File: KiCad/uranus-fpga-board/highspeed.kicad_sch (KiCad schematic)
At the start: 1 part, among them J1 ASP-134488-01

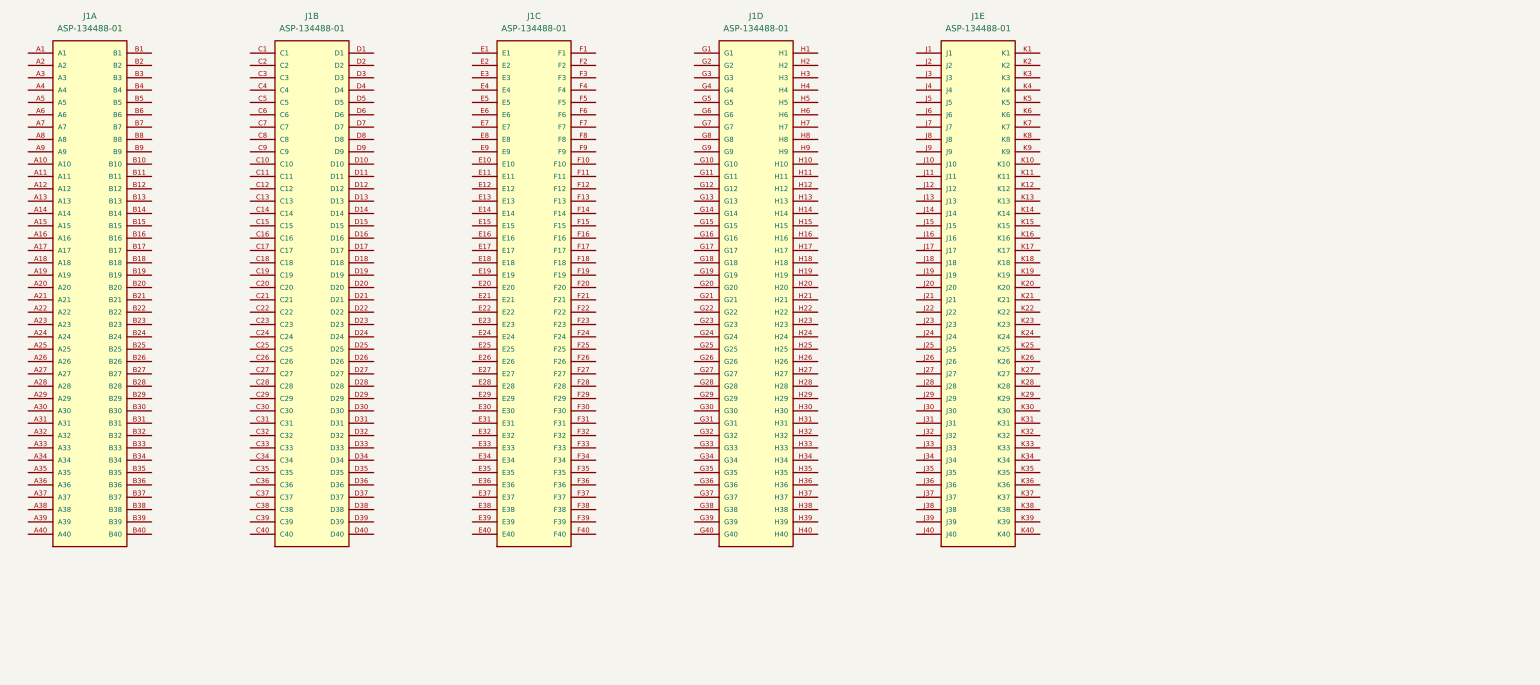
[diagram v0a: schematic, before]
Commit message: up to dating
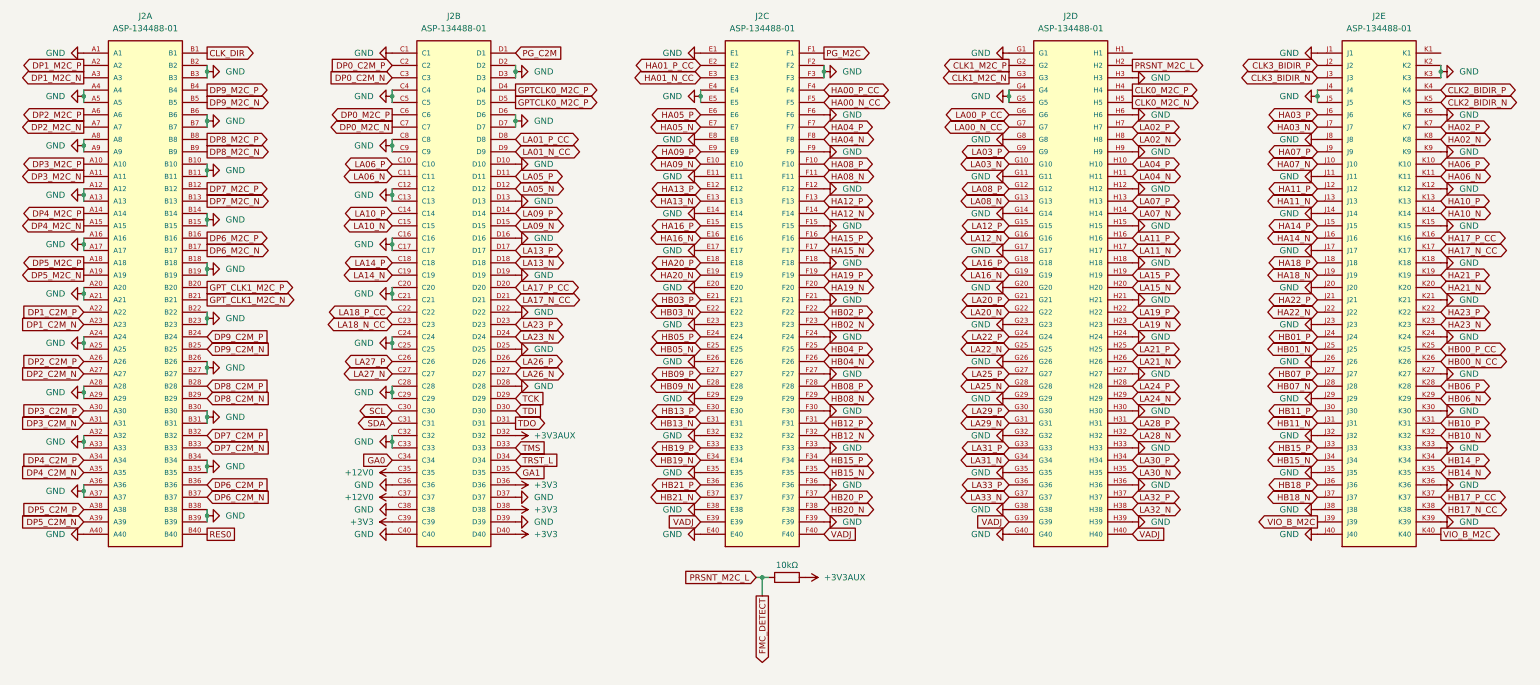
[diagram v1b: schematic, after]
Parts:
- removed J1: ASP-134488-01, FMC-HPC:SAMTEC_ASP-134488-01, symbol ASP-134488-01:ASP-134488-01
- added J2: ASP-134488-01, ASP-134488-01:SAMTEC_ASP-134488-01, symbol ASP-134488-01:ASP-134488-01
- added R14: 10kΩ, ASP-134488-01:SAMTEC_ASP-134488-01, symbol Device:R
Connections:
- new net +12V0: J2.C35, J2.C37
- new net +3V3: J2.C39, J2.D36, J2.D38, J2.D40
- new net +3V3AUX: J2.D32, R14.2
- new net CLK0_M2C_N: J2.H5
- new net CLK0_M2C_P: J2.H4
- new net CLK1_M2C_N: J2.G3
- new net CLK1_M2C_P: J2.G2
- new net CLK2_BIDIR_N: J2.K5
- new net CLK2_BIDIR_P: J2.K4
- new net CLK3_BIDIR_N: J2.J3
- new net CLK3_BIDIR_P: J2.J2
- new net CLK_DIR: J2.B1
- new net DP0_C2M_N: J2.C3
- new net DP0_C2M_P: J2.C2
- new net DP0_M2C_N: J2.C7
- new net DP0_M2C_P: J2.C6
- new net DP1_C2M_N: J2.A23
- new net DP1_C2M_P: J2.A22
- new net DP1_M2C_N: J2.A3
- new net DP1_M2C_P: J2.A2
- new net DP2_C2M_N: J2.A27
- new net DP2_C2M_P: J2.A26
- new net DP2_M2C_N: J2.A7
- new net DP2_M2C_P: J2.A6
- new net DP3_C2M_N: J2.A31
- new net DP3_C2M_P: J2.A30
- new net DP3_M2C_N: J2.A11
- new net DP3_M2C_P: J2.A10
- new net DP4_C2M_N: J2.A35
- new net DP4_C2M_P: J2.A34
- new net DP4_M2C_N: J2.A15
- new net DP4_M2C_P: J2.A14
- new net DP5_C2M_N: J2.A39
- new net DP5_C2M_P: J2.A38
- new net DP5_M2C_N: J2.A19
- new net DP5_M2C_P: J2.A18
- new net DP6_C2M_N: J2.B37
- new net DP6_C2M_P: J2.B36
- new net DP6_M2C_N: J2.B17
- new net DP6_M2C_P: J2.B16
- new net DP7_C2M_N: J2.B33
- new net DP7_C2M_P: J2.B32
- new net DP7_M2C_N: J2.B13
- new net DP7_M2C_P: J2.B12
- new net DP8_C2M_N: J2.B29
- new net DP8_C2M_P: J2.B28
- new net DP8_M2C_N: J2.B9
- new net DP8_M2C_P: J2.B8
- new net DP9_C2M_N: J2.B25
- new net DP9_C2M_P: J2.B24
- new net DP9_M2C_N: J2.B5
- new net DP9_M2C_P: J2.B4
- new net FMC_DETECT: J2.H2, R14.1
- new net GA0: J2.C34
- new net GA1: J2.D35
- new net GND: J2.A1, J2.A12, J2.A13, J2.A16, J2.A17, J2.A20, J2.A21, J2.A24, J2.A25, J2.A28, J2.A29, J2.A32, J2.A33, J2.A36, J2.A37, J2.A4, J2.A40, J2.A5, J2.A8, J2.A9, J2.B10, J2.B11, J2.B14, J2.B15, J2.B18, J2.B19, J2.B2, J2.B22, J2.B23, J2.B26, J2.B27, J2.B3, J2.B30, J2.B31, J2.B34, J2.B35, J2.B38, J2.B39, J2.B6, J2.B7, J2.C1, J2.C12, J2.C13, J2.C16, J2.C17, J2.C20, J2.C21, J2.C24, J2.C25, J2.C28, J2.C29, J2.C32, J2.C33, J2.C36, J2.C38, J2.C4, J2.C40, J2.C5, J2.C8, J2.C9, J2.D10, J2.D13, J2.D16, J2.D19, J2.D2, J2.D22, J2.D25, J2.D28, J2.D3, J2.D37, J2.D39, J2.D6, J2.D7, J2.E1, J2.E11, J2.E14, J2.E17, J2.E20, J2.E23, J2.E26, J2.E29, J2.E32, J2.E35, J2.E38, J2.E4, J2.E40, J2.E5, J2.E8, J2.F12, J2.F15, J2.F18, J2.F2, J2.F21, J2.F24, J2.F27, J2.F3, J2.F30, J2.F33, J2.F36, J2.F39, J2.F6, J2.F9, J2.G1, J2.G11, J2.G14, J2.G17, J2.G20, J2.G23, J2.G26, J2.G29, J2.G32, J2.G35, J2.G38, J2.G4, J2.G40, J2.G5, J2.G8, J2.H12, J2.H15, J2.H18, J2.H21, J2.H24, J2.H27, J2.H3, J2.H30, J2.H33, J2.H36, J2.H39, J2.H6, J2.H9, J2.J1, J2.J11, J2.J14, J2.J17, J2.J20, J2.J23, J2.J26, J2.J29, J2.J32, J2.J35, J2.J38, J2.J4, J2.J40, J2.J5, J2.J8, J2.K12, J2.K15, J2.K18, J2.K2, J2.K21, J2.K24, J2.K27, J2.K3, J2.K30, J2.K33, J2.K36, J2.K39, J2.K6, J2.K9
- new net GPTCLK0_M2C_P: J2.D4, J2.D5
- new net GPT_CLK1_M2C_N: J2.B21
- new net GPT_CLK1_M2C_P: J2.B20
- new net HA00_N_CC: J2.F5
- new net HA00_P_CC: J2.F4
- new net HA01_N_CC: J2.E3
- new net HA01_P_CC: J2.E2
- new net HA02_N: J2.K8
- new net HA02_P: J2.K7
- new net HA03_N: J2.J7
- new net HA03_P: J2.J6
- new net HA04_N: J2.F8
- new net HA04_P: J2.F7
- new net HA05_N: J2.E7
- new net HA05_P: J2.E6
- new net HA06_N: J2.K11
- new net HA06_P: J2.K10
- new net HA07_N: J2.J10
- new net HA07_P: J2.J9
- new net HA08_N: J2.F11
- new net HA08_P: J2.F10
- new net HA09_N: J2.E10
- new net HA09_P: J2.E9
- new net HA10_N: J2.K14
- new net HA10_P: J2.K13
- new net HA11_N: J2.J13
- new net HA11_P: J2.J12
- new net HA12_N: J2.F14
- new net HA12_P: J2.F13
- new net HA13_N: J2.E13
- new net HA13_P: J2.E12
- new net HA14_N: J2.J16
- new net HA14_P: J2.J15
- new net HA15_N: J2.F17
- new net HA15_P: J2.F16
- new net HA16_N: J2.E16
- new net HA16_P: J2.E15
- new net HA17_N_CC: J2.K17
- new net HA17_P_CC: J2.K16
- new net HA18_N: J2.J19
- new net HA18_P: J2.J18
- new net HA19_N: J2.F20
- new net HA19_P: J2.F19
- new net HA20_N: J2.E19
- new net HA20_P: J2.E18
- new net HA21_N: J2.K20
- new net HA21_P: J2.K19
- new net HA22_N: J2.J22
- new net HA22_P: J2.J21
- new net HA23_N: J2.K23
- new net HA23_P: J2.K22
- new net HB00_N_CC: J2.K26
- new net HB00_P_CC: J2.K25
- new net HB01_N: J2.J25
- new net HB01_P: J2.J24
- new net HB02_N: J2.F23
- new net HB02_P: J2.F22
- new net HB03_N: J2.E22
- new net HB03_P: J2.E21
- new net HB04_N: J2.F26
- new net HB04_P: J2.F25
- new net HB05_N: J2.E25
- new net HB05_P: J2.E24
- new net HB06_N: J2.K29
- new net HB06_P: J2.K28
- new net HB07_N: J2.J28
- new net HB07_P: J2.J27
- new net HB08_N: J2.F29
- new net HB08_P: J2.F28
- new net HB09_N: J2.E28
- new net HB09_P: J2.E27
- new net HB10_N: J2.K32
- new net HB10_P: J2.K31
- new net HB11_N: J2.J31
- new net HB11_P: J2.J30
- new net HB12_N: J2.F32
- new net HB12_P: J2.F31
- new net HB13_N: J2.E31
- new net HB13_P: J2.E30
- new net HB14_N: J2.K35
- new net HB14_P: J2.K34
- new net HB15_N: J2.F35, J2.J34
- new net HB15_P: J2.F34, J2.J33
- new net HB17_N_CC: J2.K38
- new net HB17_P_CC: J2.K37
- new net HB18_N: J2.J37
- new net HB18_P: J2.J36
- new net HB19_N: J2.E34
- new net HB19_P: J2.E33
- new net HB20_N: J2.F38
- new net HB20_P: J2.F37
- new net HB21_N: J2.E37
- new net HB21_P: J2.E36
- new net LA00_N_CC: J2.G7
- new net LA00_P_CC: J2.G6
- new net LA01_N_CC: J2.D9
- new net LA01_P_CC: J2.D8
- new net LA02_N: J2.H8
- new net LA02_P: J2.H7
- new net LA03_N: J2.G10
- new net LA03_P: J2.G9
- new net LA04_N: J2.H11
- new net LA04_P: J2.H10
- new net LA05_N: J2.D12
- new net LA05_P: J2.D11
- new net LA06_N: J2.C11
- new net LA06_P: J2.C10
- new net LA07_N: J2.H14
- new net LA07_P: J2.H13
- new net LA08_N: J2.G13
- new net LA08_P: J2.G12
- new net LA09_N: J2.D15
- new net LA09_P: J2.D14
- new net LA10_N: J2.C15
- new net LA10_P: J2.C14
- new net LA11_N: J2.H17
- new net LA11_P: J2.H16
- new net LA12_N: J2.G16
- new net LA12_P: J2.G15
- new net LA13_N: J2.D18
- new net LA13_P: J2.D17
- new net LA14_N: J2.C19
- new net LA14_P: J2.C18
- new net LA15_N: J2.H20
- new net LA15_P: J2.H19
- new net LA16_N: J2.G19
- new net LA16_P: J2.G18
- new net LA17_N_CC: J2.D21
- new net LA17_P_CC: J2.D20
- new net LA18_N_CC: J2.C23
- new net LA18_P_CC: J2.C22
- new net LA19_N: J2.H23
- new net LA19_P: J2.H22
- new net LA20_N: J2.G22
- new net LA20_P: J2.G21
- new net LA21_N: J2.H26
- new net LA21_P: J2.H25
- new net LA22_N: J2.G25
- new net LA22_P: J2.G24
- new net LA23_N: J2.D24
- new net LA23_P: J2.D23
- new net LA24_N: J2.H29
- new net LA24_P: J2.H28
- new net LA25_N: J2.G28
- new net LA25_P: J2.G27
- new net LA26_N: J2.D27
- new net LA26_P: J2.D26
- new net LA27_N: J2.C27
- new net LA27_P: J2.C26
- new net LA28_N: J2.H32
- new net LA28_P: J2.H31
- new net LA29_N: J2.G31
- new net LA29_P: J2.G30
- new net LA30_N: J2.H35
- new net LA30_P: J2.H34
- new net LA31_N: J2.G34
- new net LA31_P: J2.G33
- new net LA32_N: J2.H38
- new net LA32_P: J2.H37
- new net LA33_N: J2.G37
- new net LA33_P: J2.G36
- new net PG_C2M: J2.D1
- new net PG_M2C: J2.F1
- new net RES0: J2.B40
- new net SCL: J2.C30
- new net SDA: J2.C31
- new net TCK: J2.D29
- new net TDI: J2.D30
- new net TDO: J2.D31
- new net TMS: J2.D33
- new net TRST_L: J2.D34
- new net VADJ: J2.E39, J2.F40, J2.G39, J2.H40
- new net VIO_B_M2C: J2.J39, J2.K40
